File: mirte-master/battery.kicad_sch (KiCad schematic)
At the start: 2 parts, among them J15 batt_xt90, J16 batt_deans

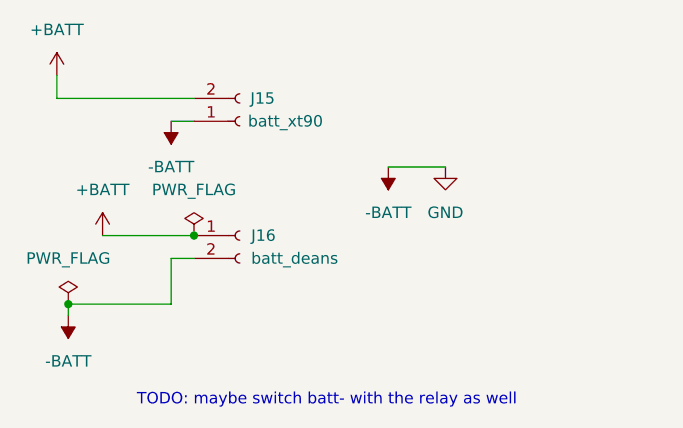
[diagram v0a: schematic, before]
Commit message: Shrunk and cleanup
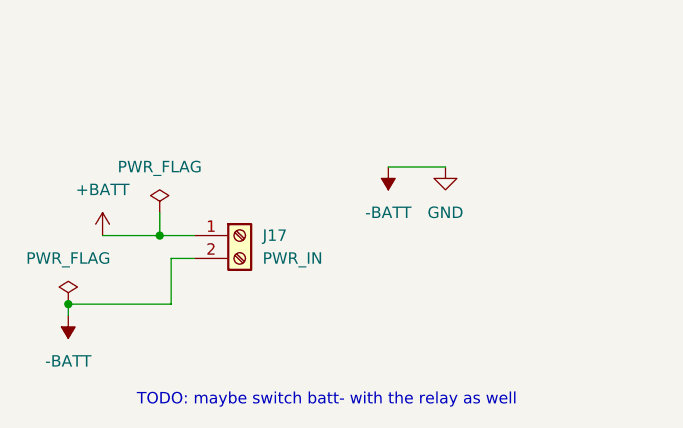
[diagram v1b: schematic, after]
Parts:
- removed J15: batt_xt90, xt90:AMASS_XT90-F_1x02_P11.00mm_Vertical, symbol Connector:Conn_01x02_Socket
- removed J16: batt_deans, xt90:DEANS, symbol Connector:Conn_01x02_Socket
- added J17: PWR_IN, TerminalBlock_Phoenix:TerminalBlock_Phoenix_PT-1,5-2-5.0-H_1x02_P5.00mm_Horizontal, symbol Connector:Screw_Terminal_01x02
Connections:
- net +BATT: now also J17.1 (Pin_1)
- net -BATT: now also J17.2 (Pin_2)
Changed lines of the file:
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@@
 (kicad_sch (version 20230121) (generator eeschema)
   (paper "A4")
+  (junction (at 45.72 78.74) (diameter 0) (color 0 0 0 0)
+  )
   (junction (at 35.56 86.36) (diameter 0) (color 0 0 0 0)
   )
-  (junction (at 49.53 78.74) (diameter 0) (color 0 0 0 0)
-  )
-  (wire (pts (xy 39.37 78.74) (xy 49.53 78.74))
+  (wire (pts (xy 39.37 78.74) (xy 45.72 78.74))
     (stroke (width 0) (type default))
   )
@@
     (stroke (width 0) (type default))
   )
-  (wire (pts (xy 49.53 66.04) (xy 46.99 66.04))
+  (wire (pts (xy 45.72 78.74) (xy 49.53 78.74))
     (stroke (width 0) (type default))
   )
-  (wire (pts (xy 34.29 63.5) (xy 34.29 60.96))
-    (stroke (width 0) (type default))
-  )
-  (wire (pts (xy 34.29 63.5) (xy 49.53 63.5))
+  (wire (pts (xy 45.72 76.2) (xy 45.72 78.74))
     (stroke (width 0) (type default))
   )
@@
     )
   )
-  (symbol (lib_id "Connector:Conn_01x02_Socket") (at 54.61 78.74 0) (unit 1)
-    (in_bom yes) (on_board yes) (dnp no) (fields_autoplaced)
-    (property "Reference" "J16" (at 55.88 78.74 0)
-      (effects (font (size 1.27 1.27)) (justify left))
-    )
-    (property "Value" "batt_deans" (at 55.88 81.28 0)
-      (effects (font (size 1.27 1.27)) (justify left))
-    )
-    (property "Footprint" "xt90:DEANS" (at 54.61 78.74 0)
-      (effects (font (size 1.27 1.27)) hide)
-    )
-    (property "Datasheet" "~" (at 54.61 78.74 0)
-      (effects (font (size 1.27 1.27)) hide)
-    )
-    (pin "2")
-    (pin "1")
-    (instances
-      (project "mirte-master"
-        (path "/19794465-0368-488c-958e-83b02754ebd6/17ebe4c8-09bb-4699-976c-396d27e4a3f5/1289cdbf-c89c-46a5-93db-3249bdca7927"
-          (reference "J16") (unit 1)
-        )
-      )
-    )
-  )
   (symbol (lib_id "power:GND") (at 77.47 71.12 0) (unit 1)
     (in_bom yes) (on_board yes) (dnp no) (fields_autoplaced)
@@
     )
   )
-  (symbol (lib_id "power:-BATT") (at 46.99 66.04 180) (unit 1)
-    (in_bom yes) (on_board yes) (dnp no) (fields_autoplaced)
-    (property "Reference" "#PWR033" (at 46.99 62.23 0)
+  (symbol (lib_id "Connector:Screw_Terminal_01x02") (at 54.61 78.74 0) (unit 1)
+    (in_bom yes) (on_board yes) (dnp no)
+    (property "Reference" "J17" (at 57.15 78.74 0)
+      (effects (font (size 1.27 1.27)) (justify left))
+    )
+    (property "Value" "PWR_IN" (at 57.15 81.28 0)
+      (effects (font (size 1.27 1.27)) (justify left))
+    )
+    (property "Footprint" "TerminalBlock_Phoenix:TerminalBlock_Phoenix_PT-1,5-2-5.0-H_1x02_P5.00mm_Horizontal" (at 54.61 78.74 0)
       (effects (font (size 1.27 1.27)) hide)
     )
-    (property "Value" "-BATT" (at 46.99 71.12 0)
-      (effects (font (size 1.27 1.27)))
-    )
-    (property "Footprint" "" (at 46.99 66.04 0)
+    (property "Datasheet" "~" (at 54.61 78.74 0)
       (effects (font (size 1.27 1.27)) hide)
     )
-    (property "Datasheet" "" (at 46.99 66.04 0)
-      (effects (font (size 1.27 1.27)) hide)
-    )
+    (pin "2")
     (pin "1")
     (instances
       (project "mirte-master"
+        (path "/19794465-0368-488c-958e-83b02754ebd6/17ebe4c8-09bb-4699-976c-396d27e4a3f5/544a16a8-9ef3-43b3-aa0f-4bd972816cae/d3337f2d-26a9-4529-9bfc-380e6deefc08"
+          (reference "J17") (unit 1)
+        )
         (path "/19794465-0368-488c-958e-83b02754ebd6/17ebe4c8-09bb-4699-976c-396d27e4a3f5/1289cdbf-c89c-46a5-93db-3249bdca7927"
-          (reference "#PWR033") (unit 1)
+          (reference "J15") (unit 1)
         )
       )
     )
   )
-  (symbol (lib_id "power:PWR_FLAG") (at 49.53 78.74 0) (unit 1)
+  (symbol (lib_id "power:PWR_FLAG") (at 45.72 76.2 0) (unit 1)
     (in_bom yes) (on_board yes) (dnp no) (fields_autoplaced)
-    (property "Reference" "#FLG02" (at 49.53 76.835 0)
+    (property "Reference" "#FLG02" (at 45.72 74.295 0)
       (effects (font (size 1.27 1.27)) hide)
     )
-    (property "Value" "PWR_FLAG" (at 49.53 73.66 0)
+    (property "Value" "PWR_FLAG" (at 45.72 71.12 0)
       (effects (font (size 1.27 1.27)))
     )
-    (property "Footprint" "" (at 49.53 78.74 0)
+    (property "Footprint" "" (at 45.72 76.2 0)
       (effects (font (size 1.27 1.27)) hide)
     )
-    (property "Datasheet" "~" (at 49.53 78.74 0)
+    (property "Datasheet" "~" (at 45.72 76.2 0)
       (effects (font (size 1.27 1.27)) hide)
     )
@@
         )
       )
-    )
-  )
-  (symbol (lib_id "Connector:Conn_01x02_Socket") (at 54.61 66.04 0) (mirror x) (unit 1)
-    (in_bom yes) (on_board yes) (dnp no)
-    (property "Reference" "J15" (at 57.15 63.5 0)
-      (effects (font (size 1.27 1.27)))
-    )
-    (property "Value" "batt_xt90" (at 59.69 66.04 0)
-      (effects (font (size 1.27 1.27)))
-    )
-    (property "Footprint" "xt90:AMASS_XT90-F_1x02_P11.00mm_Vertical" (at 54.61 66.04 0)
-      (effects (font (size 1.27 1.27)) hide)
-    )
-    (property "Datasheet" "~" (at 54.61 66.04 0)
-      (effects (font (size 1.27 1.27)) hide)
-    )
-    (pin "2")
-    (pin "1")
-    (instances
-      (project "mirte-master"
-        (path "/19794465-0368-488c-958e-83b02754ebd6/17ebe4c8-09bb-4699-976c-396d27e4a3f5/1289cdbf-c89c-46a5-93db-3249bdca7927"
-          (reference "J15") (unit 1)
-        )
-      )
-    )
-  )
-  (symbol (lib_id "power:+BATT") (at 34.29 60.96 0) (unit 1)
-    (in_bom yes) (on_board yes) (dnp no) (fields_autoplaced)
-    (property "Reference" "#PWR035" (at 34.29 64.77 0)
-      (effects (font (size 1.27 1.27)) hide)
-    )
-    (property "Value" "+BATT" (at 34.29 55.88 0)
-      (effects (font (size 1.27 1.27)))
-    )
-    (property "Footprint" "" (at 34.29 60.96 0)
-      (effects (font (size 1.27 1.27)) hide)
-    )
-    (property "Datasheet" "" (at 34.29 60.96 0)
-      (effects (font (size 1.27 1.27)) hide)
-    )
-    (pin "1")
-    (instances
-      (project "mirte-master"
-        (path "/19794465-0368-488c-958e-83b02754ebd6/17ebe4c8-09bb-4699-976c-396d27e4a3f5/1289cdbf-c89c-46a5-93db-3249bdca7927"
-          (reference "#PWR035") (unit 1)
-        )
-      )
